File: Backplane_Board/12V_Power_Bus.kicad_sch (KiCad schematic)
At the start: 14 parts, among them U5 PKU3511SPI

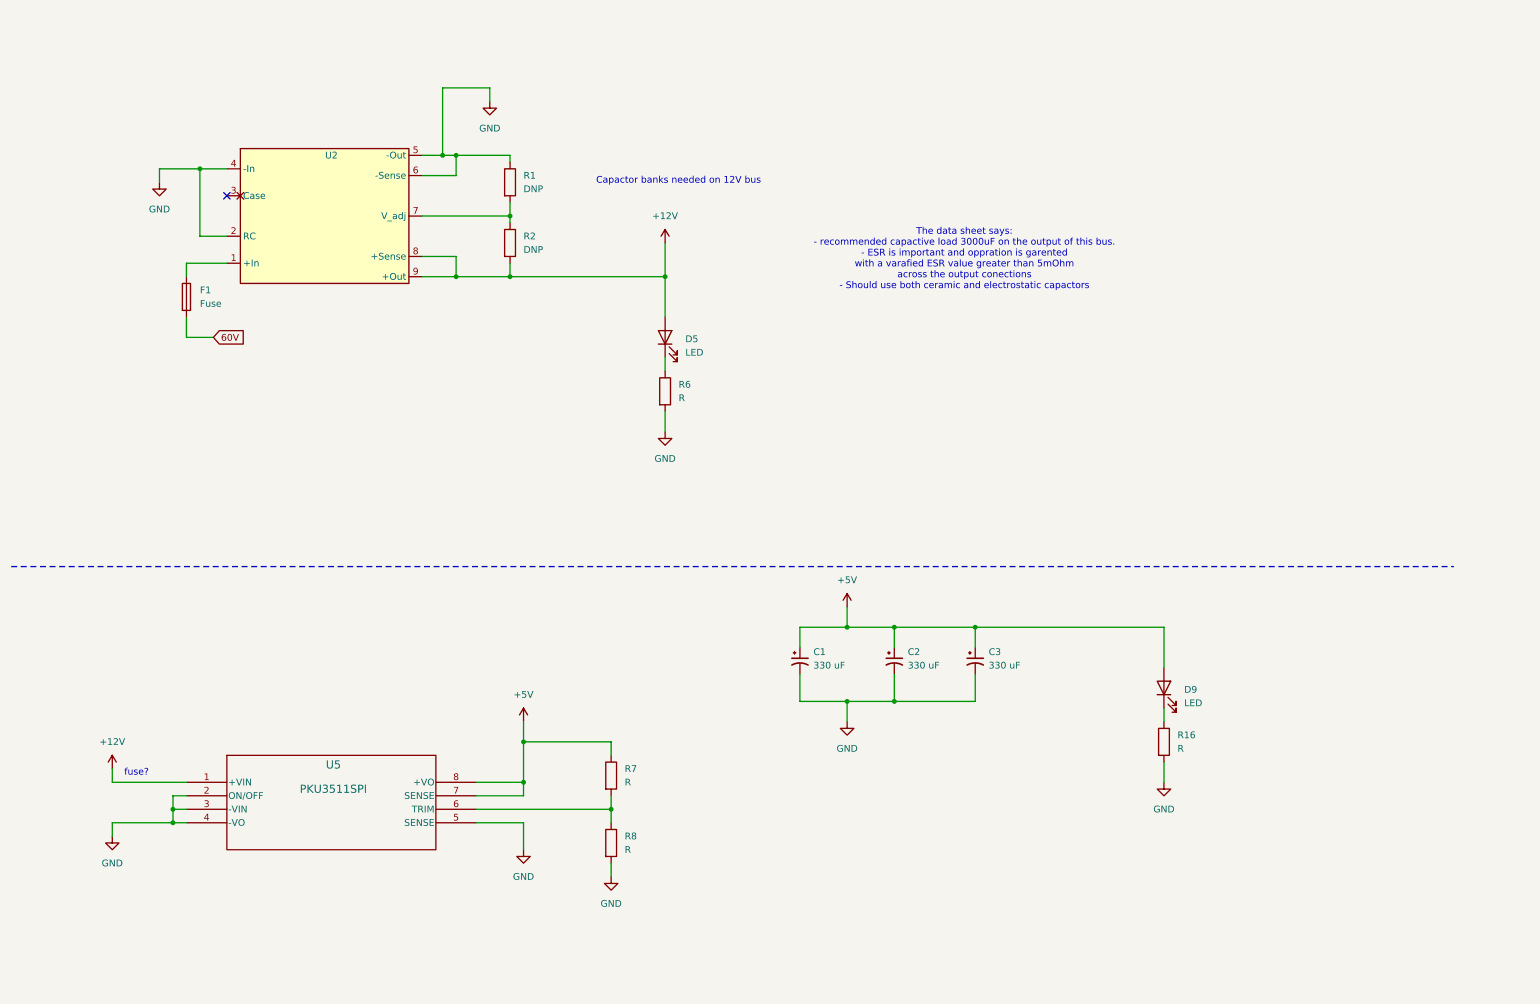
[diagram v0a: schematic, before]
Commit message: back plane board ready for review
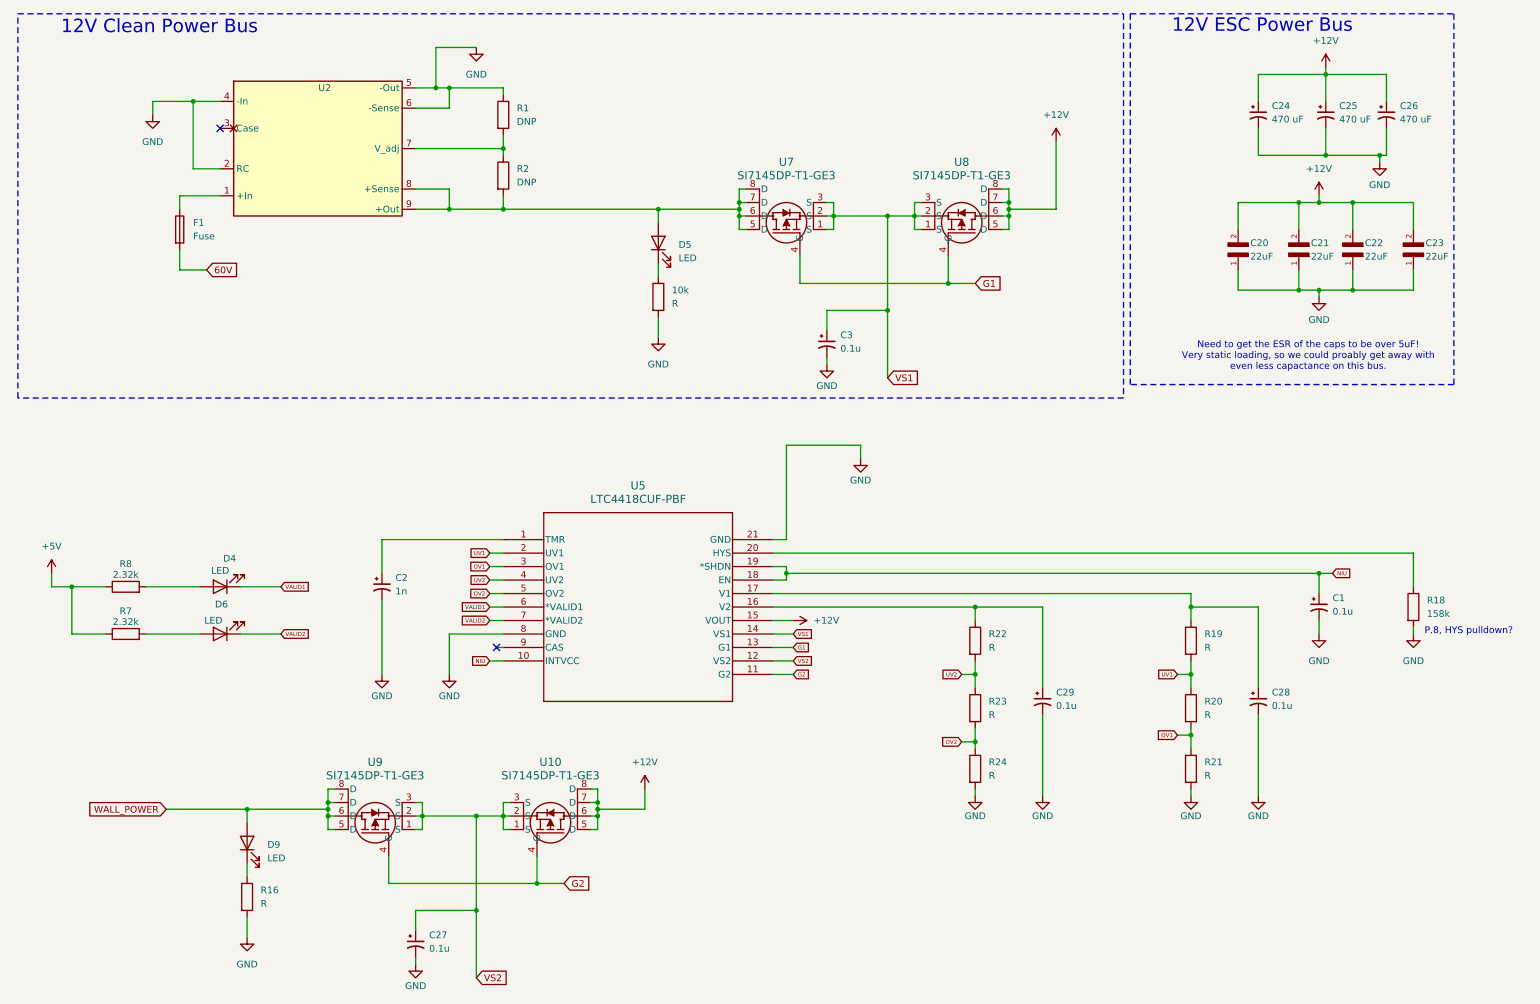
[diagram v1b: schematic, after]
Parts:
- removed U5: PKU3511SPI, PKU 3500S_FPM, symbol PKU3511SPI:PKU3511SPI
- added C20, C21, C22, C23: 22uF, C2012X5R1V226M125AC:CAPC2012X145N, symbol C2012X5R1V226M125AC:C2012X5R1V226M125AC
- added C24, C25, C26: 470 uF, 470UF CAP:CAP_EEHZU1V471V, symbol Device:C_Polarized_Small_US
- added C27, C28, C29: 0.1u, symbol Device:C_Polarized_Small_US
- added D4, D6: LED, symbol Device:LED
- added R18: 158k, symbol Device:R
- added R19, R20, R21, R22, R23, R24: R, symbol Device:R
- added U10, U7, U8, U9: SI7145DP-T1-GE3, SON8_SI7135DP-T1-GE3_VIS, symbol SI7145DP_T1_GE3:SI7145DP-T1-GE3
- added U5: LTC4418CUF-PBF, UF_20_ADI, symbol ul_LTC4418CUF-PBF:LTC4418CUF-PBF
- C1, C3: value 330 uF -> 0.1u; footprint 220UF CAP:CAP_16SVPG330MX -> (none)
- C2: value 330 uF -> 1n; footprint 220UF CAP:CAP_16SVPG330MX -> (none)
- R7, R8: value R -> 2.32k
- renumbered R6 to 10k
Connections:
- net +12V: now also C20.2, C21.2, C22.2, C23.2, C24.1, C25.1, C26.1, U10.5 (D), U10.6 (D), U10.7 (D), U10.8 (D), U5.15 (VOUT), U8.5 (D), U8.6 (D), U8.7 (D), U8.8 (D); no longer D5.2 (A), R2.2, U2.8 (+Sense), U2.9 (+Out)
- net +5V: now also R8.1; no longer C1.1, C2.1, C3.1, D9.2 (A)
- net GND: now also C20.1, C21.1, C22.1, C23.1, C24.2, C25.2, C26.2, C27.2, C28.2, C29.2, R18.2, R21.2, R24.2, U5.21 (GND), U5.8 (GND); no longer R8.2
- net at R7.2: now also D6.2 (A); no longer R8.1
- new net: C28.1, R19.1, U5.17 (V1)
- new net: C29.1, R22.1, U5.16 (V2)
- new net: C2.1, U5.1 (TMR)
- new net: D5.2 (A), R2.2, U2.8 (+Sense), U2.9 (+Out), U7.5 (D), U7.6 (D), U7.7 (D), U7.8 (D)
- new net: R18.1, U5.20 (HYS)
- new net: D4.2 (A), R8.2
- new net G1: U5.13 (G1), U7.4 (G), U8.4 (G)
- new net G2: U10.4 (G), U5.11 (G2), U9.4 (G)
- new net NIU: C1.1, U5.10 (INTVCC), U5.18 (EN), U5.19 (*SHDN)
- new net OV1: R20.2, R21.1, U5.3 (OV1)
- new net OV2: R23.2, R24.1, U5.5 (OV2)
- new net UV1: R19.2, R20.1, U5.2 (UV1)
- new net UV2: R22.2, R23.1, U5.4 (UV2)
- new net VALID1: D4.1 (K), U5.6 (*VALID1)
- new net VALID2: D6.1 (K), U5.7 (*VALID2)
- new net VS1: C3.1, U5.14 (VS1), U7.1 (S), U7.2 (S), U7.3 (S), U8.1 (S), U8.2 (S), U8.3 (S)
- new net VS2: C27.1, U10.1 (S), U10.2 (S), U10.3 (S), U5.12 (VS2), U9.1 (S), U9.2 (S), U9.3 (S)
- new net WALL_POWER: D9.2 (A), U9.5 (D), U9.6 (D), U9.7 (D), U9.8 (D)
- no-connect marks 1 -> 2
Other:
- note added: "12V Clean Power Bus"
- note added: "12V ESC Power Bus"
- note added: "Need to get the ESR of the caps to be over 5uF! Very static loading, so we could proably get away with even less capactance on this bus."
- note added: "P.8, HYS pulldown?"
- note removed: "Capactor banks needed on 12V bus"
- note removed: "The data sheet says: - recommended capactive load 3000uF on the output of this bus. - ESR is important and oppration is garented with a varafied ESR value greater than 5mOhm across the output conections - Should use both ceramic and electrostatic capactors"
- note removed: "fuse?"
- moved on the sheet: 10k, D5, F1, R1, R2, U2
